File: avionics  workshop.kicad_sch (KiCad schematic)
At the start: 12 parts, among them U1 BMP280, U4 AMS1117-3.3

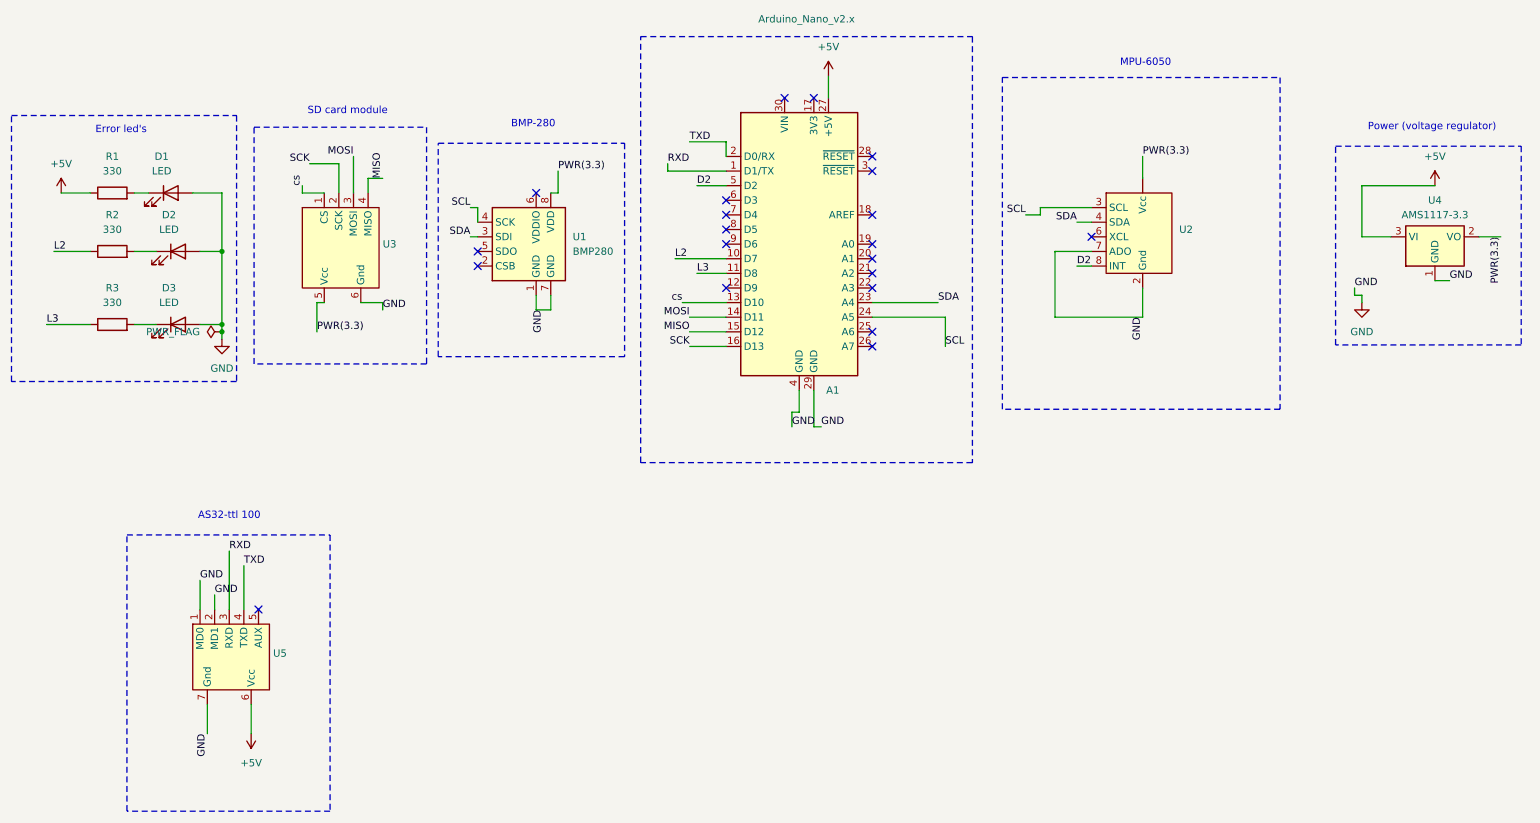
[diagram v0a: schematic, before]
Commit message: draft7
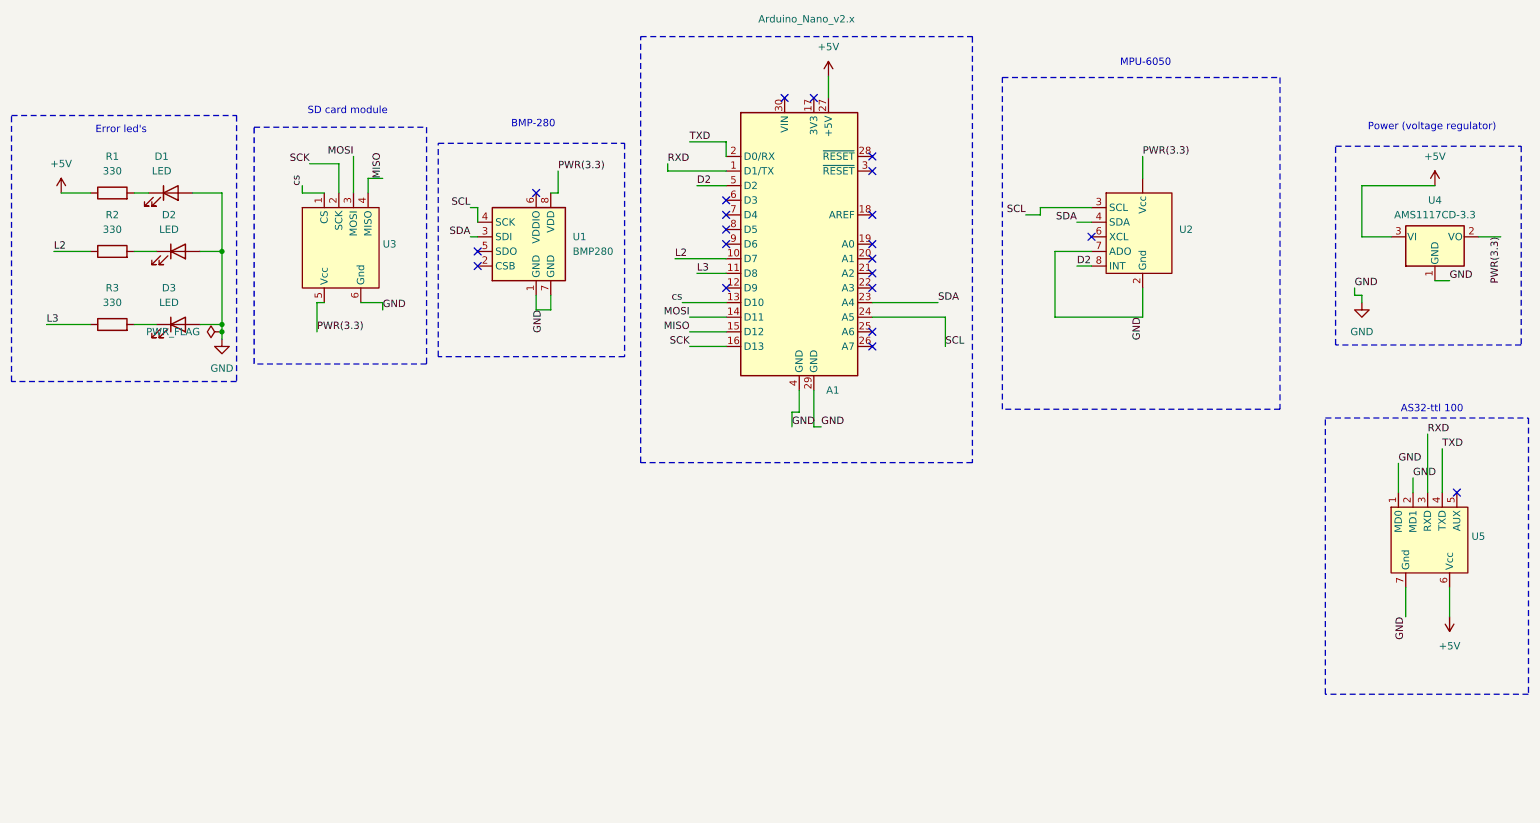
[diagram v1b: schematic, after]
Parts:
- removed U4: AMS1117-3.3, Package_TO_SOT_SMD:SOT-223-3_TabPin2, symbol Regulator_Linear:AMS1117-3.3
- added U4: AMS1117CD-3.3, GovindLibrary:AMS-1117, symbol Regulator_Linear:AMS1117CD-3.3
- U1: footprint Package_LGA:Bosch_LGA-8_2x2.5mm_P0.65mm_ClockwisePinNumbering -> GovindLibrary:BMP280
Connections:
- net +5V: now also U4.3 (VI)
- net GND: now also U4.1 (GND)
- net PWR(3.3): now also U4.2 (VO)
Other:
- moved on the sheet: U5
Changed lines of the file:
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@@
 	)
 	(rectangle
-		(start 35.56 133.096)
-		(end 70.866 181.102)
+		(start 243.84 112.776)
+		(end 279.146 160.782)
 		(stroke
 			(width 0)
@@
 	(text "AS32-ttl 100"
 		(exclude_from_sim no)
-		(at 53.34 129.794 0)
+		(at 262.382 111.252 0)
 		(effects
 			(font
@@
 	)
 	(no_connect
-		(at 58.42 146.05)
+		(at 266.7 125.73)
 	)
 	(no_connect
@@
 	(wire
 		(pts
-			(xy 55.88 138.43) (xy 55.88 146.05)
+			(xy 264.16 118.11) (xy 264.16 125.73)
 		)
 		(stroke
@@
 	(wire
 		(pts
-			(xy 53.34 135.89) (xy 53.34 146.05)
+			(xy 261.62 115.57) (xy 261.62 125.73)
 		)
 		(stroke
@@
 	(wire
 		(pts
-			(xy 48.26 140.97) (xy 48.26 146.05)
+			(xy 256.54 120.65) (xy 256.54 125.73)
 		)
 		(stroke
@@
 	(wire
 		(pts
-			(xy 57.15 162.56) (xy 57.15 167.64)
+			(xy 265.43 142.24) (xy 265.43 147.32)
 		)
 		(stroke
@@
 	(wire
 		(pts
-			(xy 49.53 162.56) (xy 49.53 167.64)
+			(xy 257.81 142.24) (xy 257.81 147.32)
 		)
 		(stroke
@@
 	(wire
 		(pts
-			(xy 50.8 143.51) (xy 50.8 146.05)
+			(xy 259.08 123.19) (xy 259.08 125.73)
 		)
 		(stroke
@@
 	)
 	(label "RXD"
-		(at 53.34 135.89 0)
+		(at 261.62 115.57 0)
 		(effects
 			(font
@@
 	)
 	(label "GND"
-		(at 49.53 167.64 270)
+		(at 257.81 147.32 270)
 		(effects
 			(font
@@
 	)
 	(label "GND"
-		(at 48.26 140.97 0)
+		(at 256.54 120.65 0)
 		(effects
 			(font
@@
 	)
 	(label "GND"
-		(at 50.8 143.51 0)
+		(at 259.08 123.19 0)
 		(effects
 			(font
@@
 	)
 	(label "TXD"
-		(at 55.88 138.43 0)
+		(at 264.16 118.11 0)
 		(effects
 			(font
@@
 	(symbol
 		(lib_id "New_Library:AS32-TTL100")
-		(at 53.34 153.67 0)
+		(at 261.62 133.35 0)
 		(unit 1)
 		(exclude_from_sim no)
@@
 		(fields_autoplaced yes)
 		(property "Reference" "U5"
-			(at 60.96 153.6699 0)
+			(at 269.24 133.3499 0)
 			(effects
 				(font
@@
 		)
 		(property "Value" "~"
-			(at 60.96 155.575 0)
+			(at 269.24 135.255 0)
 			(effects
 				(font
@@
 		)
 		(property "Footprint" "GovindLibrary:AS32-TTL100"
-			(at 53.34 153.67 0)
+			(at 261.62 133.35 0)
 			(effects
 				(font
@@
 		)
 		(property "Datasheet" ""
-			(at 53.34 153.67 0)
+			(at 261.62 133.35 0)
 			(effects
 				(font
@@
 		)
 		(property "Description" ""
-			(at 53.34 153.67 0)
+			(at 261.62 133.35 0)
 			(effects
 				(font
@@
 	(symbol
 		(lib_id "power:+5V")
-		(at 57.15 167.64 180)
+		(at 265.43 147.32 180)
 		(unit 1)
 		(exclude_from_sim no)
@@
 		(fields_autoplaced yes)
 		(property "Reference" "#PWR06"
-			(at 57.15 163.83 0)
+			(at 265.43 143.51 0)
 			(effects
 				(font
@@
 		)
 		(property "Value" "+5V"
-			(at 57.15 172.72 0)
+			(at 265.43 152.4 0)
 			(effects
 				(font
@@
 		)
 		(property "Footprint" ""
-			(at 57.15 167.64 0)
+			(at 265.43 147.32 0)
 			(effects
 				(font
@@
 		)
 		(property "Datasheet" ""
-			(at 57.15 167.64 0)
+			(at 265.43 147.32 0)
 			(effects
 				(font
@@
 		)
 		(property "Description" "Power symbol creates a global label with name \"+5V\""
-			(at 57.15 167.64 0)
+			(at 265.43 147.32 0)
 			(effects
 				(font
@@
 				(path "/b922d51f-b961-4ded-8569-767b32b1ff85"
 					(reference "A1")
-					(unit 1)
-				)
-			)
-		)
-	)
-	(symbol
-		(lib_id "Regulator_Linear:AMS1117-3.3")
-		(at 262.89 81.28 0)
-		(unit 1)
-		(exclude_from_sim no)
-		(in_bom yes)
-		(on_board yes)
-		(dnp no)
-		(fields_autoplaced yes)
-		(property "Reference" "U4"
-			(at 262.89 74.93 0)
-			(effects
-				(font
-					(size 1.27 1.27)
-				)
-			)
-		)
-		(property "Value" "AMS1117-3.3"
-			(at 262.89 77.47 0)
-			(effects
-				(font
-					(size 1.27 1.27)
-				)
-			)
-		)
-		(property "Footprint" "Package_TO_SOT_SMD:SOT-223-3_TabPin2"
-			(at 262.89 76.2 0)
-			(effects
-				(font
-					(size 1.27 1.27)
-				)
-				(hide yes)
-			)
-		)
-		(property "Datasheet" "http://www.advanced-monolithic.com/pdf/ds1117.pdf"
-			(at 265.43 87.63 0)
-			(effects
-				(font
-					(size 1.27 1.27)
-				)
-				(hide yes)
-			)
-		)
-		(property "Description" "1A Low Dropout regulator, positive, 3.3V fixed output, SOT-223"
-			(at 262.89 81.28 0)
-			(effects
-				(font
-					(size 1.27 1.27)
-				)
-				(hide yes)
-			)
-		)
-		(pin "3"
-		)
-		(pin "1"
-		)
-		(pin "2"
-		)
-		(instances
-			(project ""
-				(path "/b922d51f-b961-4ded-8569-767b32b1ff85"
-					(reference "U4")
 					(unit 1)
 				)
@@
 	)
 	(symbol
+		(lib_id "Regulator_Linear:AMS1117CD-3.3")
+		(at 262.89 81.28 0)
+		(unit 1)
+		(exclude_from_sim no)
+		(in_bom yes)
+		(on_board yes)
+		(dnp no)
+		(fields_autoplaced yes)
+		(property "Reference" "U4"
+			(at 262.89 74.93 0)
+			(effects
+				(font
+					(size 1.27 1.27)
+				)
+			)
+		)
+		(property "Value" "AMS1117CD-3.3"
+			(at 262.89 77.47 0)
+			(effects
+				(font
+					(size 1.27 1.27)
+				)
+			)
+		)
+		(property "Footprint" "GovindLibrary:AMS-1117"
+			(at 262.89 76.2 0)
+			(effects
+				(font
+					(size 1.27 1.27)
+				)
+				(hide yes)
+			)
+		)
+		(property "Datasheet" "http://www.advanced-monolithic.com/pdf/ds1117.pdf"
+			(at 265.43 87.63 0)
+			(effects
+				(font
+					(size 1.27 1.27)
+				)
+				(hide yes)
+			)
+		)
+		(property "Description" "1A Low Dropout regulator, positive, 3.3V fixed output, TO-252"
+			(at 262.89 81.28 0)
+			(effects
+				(font
+					(size 1.27 1.27)
+				)
+				(hide yes)
+			)
+		)
+		(pin "2"
+		)
+		(pin "1"
+		)
+		(pin "3"
+		)
+		(instances
+			(project ""
+				(path "/b922d51f-b961-4ded-8569-767b32b1ff85"
+					(reference "U4")
+					(unit 1)
+				)
+			)
+		)
+	)
+	(symbol
 		(lib_id "power:PWR_FLAG")
 		(at 52.07 97.79 90)
@@
 			)
 		)
-		(property "Footprint" "Package_LGA:Bosch_LGA-8_2x2.5mm_P0.65mm_ClockwisePinNumbering"
+		(property "Footprint" "GovindLibrary:BMP280"
 			(at 106.68 101.6 0)
 			(effects
